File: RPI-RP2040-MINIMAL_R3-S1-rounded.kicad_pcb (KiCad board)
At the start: 2 copper layers, 65 x 46.7 mm, 31 parts, among them J3 Conn_01x04_Pin, J4 Conn_01x04_Socket, P1 USB_C_Plug_USB2.0, U1 NCP1117ST33T3G, U2 W25Q128JVSIQ, U3 RP2040, X1 12MHz

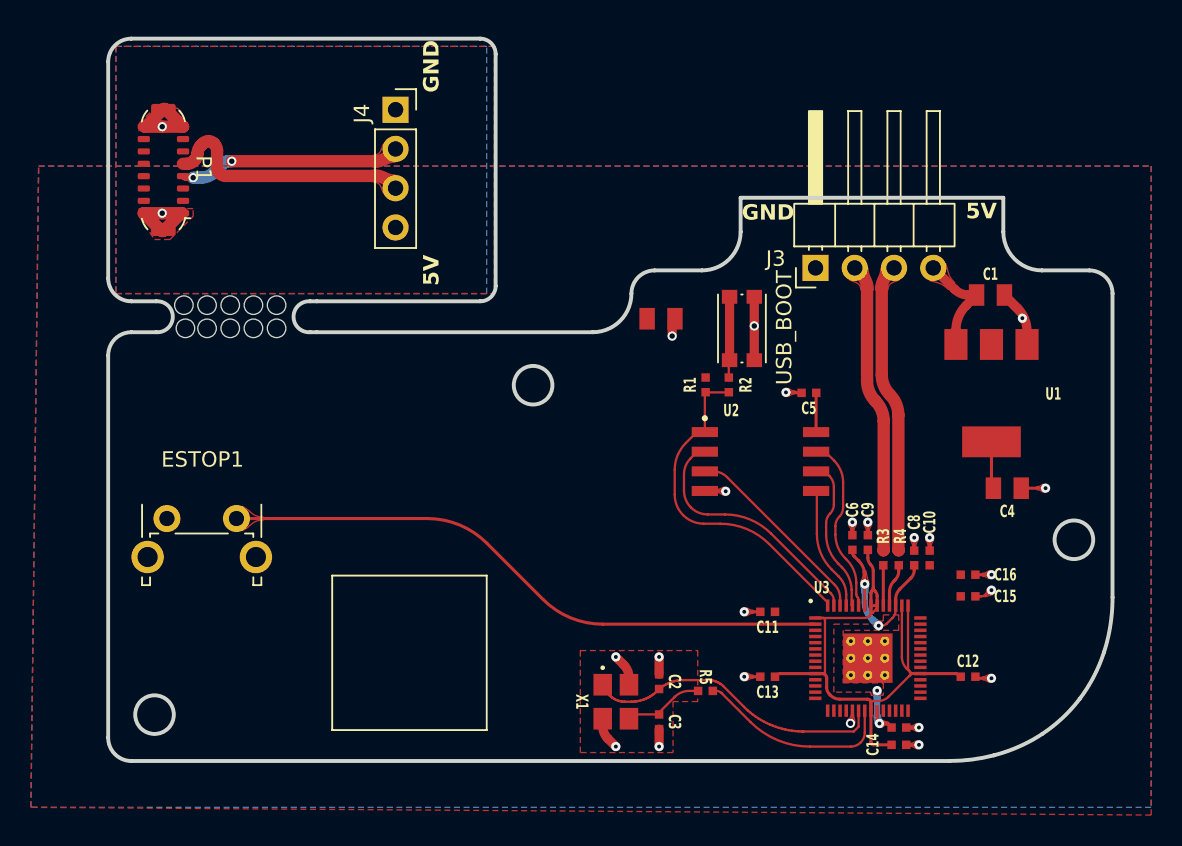
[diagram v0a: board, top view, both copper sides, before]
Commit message: Rounding
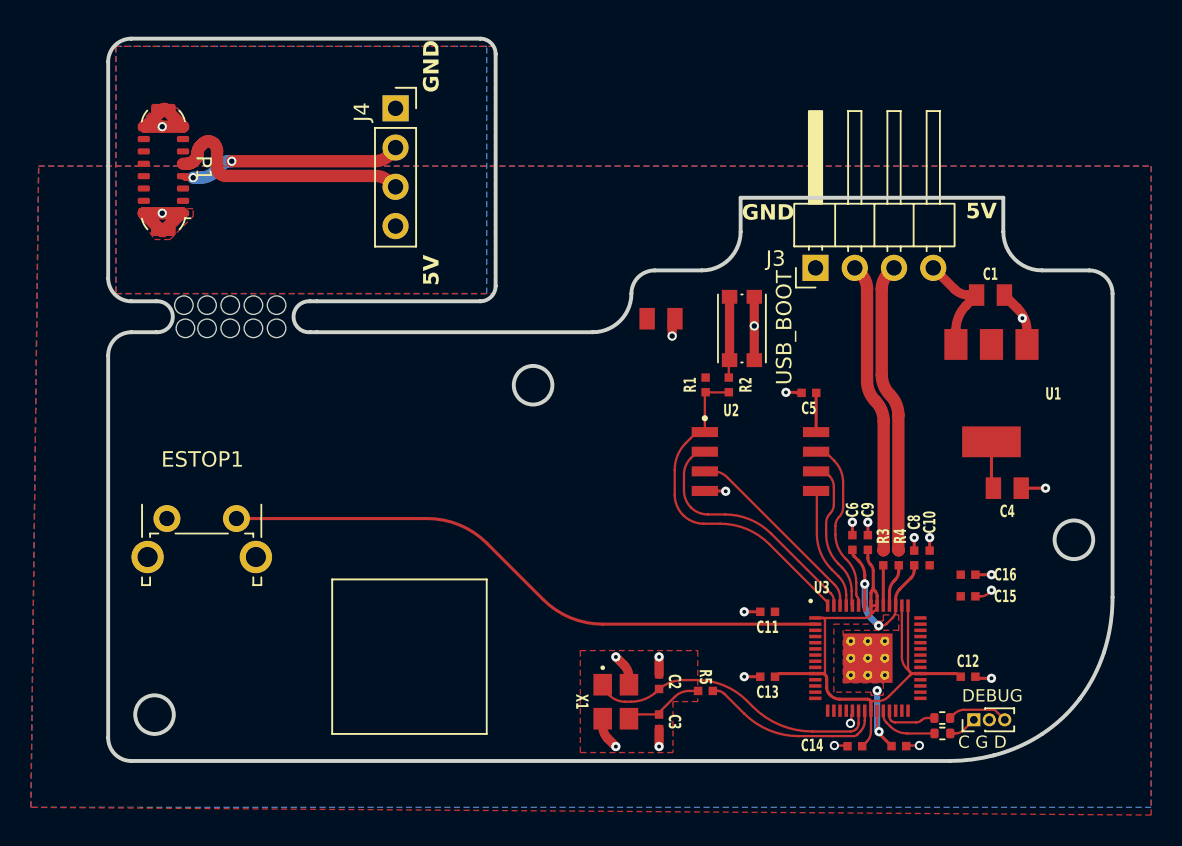
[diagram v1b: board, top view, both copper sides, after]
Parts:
- added J1: Conn_01x03_Socket, Connector_PinHeader_1.00mm:PinHeader_1x03_P1.00mm_Vertical, F.Cu at (106.5, 104.3)
- added R6: 100, Resistor_SMD:R_0402_1005Metric, F.Cu at (104.5, 105.2)
- added R7: 100, Resistor_SMD:R_0402_1005Metric, F.Cu at (104.5, 104.2)
- moved C14 2.85 mm to (98.8, 106.0), turned to 180 degrees
- moved C7 1.20 mm to (101.7, 106.0)
- moved J4 0.09 mm to (69.1, 64.8)
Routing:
- net /SWCLK: track 0.00 -> 4.15 mm
- net Net-(J1-Pin_3): track 0.00 -> 3.98 mm
- net /SWD: track 0.00 -> 3.57 mm
- net +1V1: track 15.2 -> 17.1 mm
- net Net-(J1-Pin_1): track 0.00 -> 1.86 mm
- net /BRIDGE_USBD-: track 16.6 -> 18.1 mm
- net +3V3: track 48.0 -> 47.3 mm
- net /XIN: track 19.1 -> 19.6 mm
- net /QSPI_SD2: track 12.3 -> 12.8 mm
- net /XOUT: track 12.9 -> 12.4 mm
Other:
- board text added: "C G D"
- board text added: "DEBUG"
